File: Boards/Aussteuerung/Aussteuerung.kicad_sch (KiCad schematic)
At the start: 17 parts, among them J1 6V3_Heater, J2 Signal_R, J3 Signal_R, J4 250VDC, K1 FINDER-34.51, U1 EM84

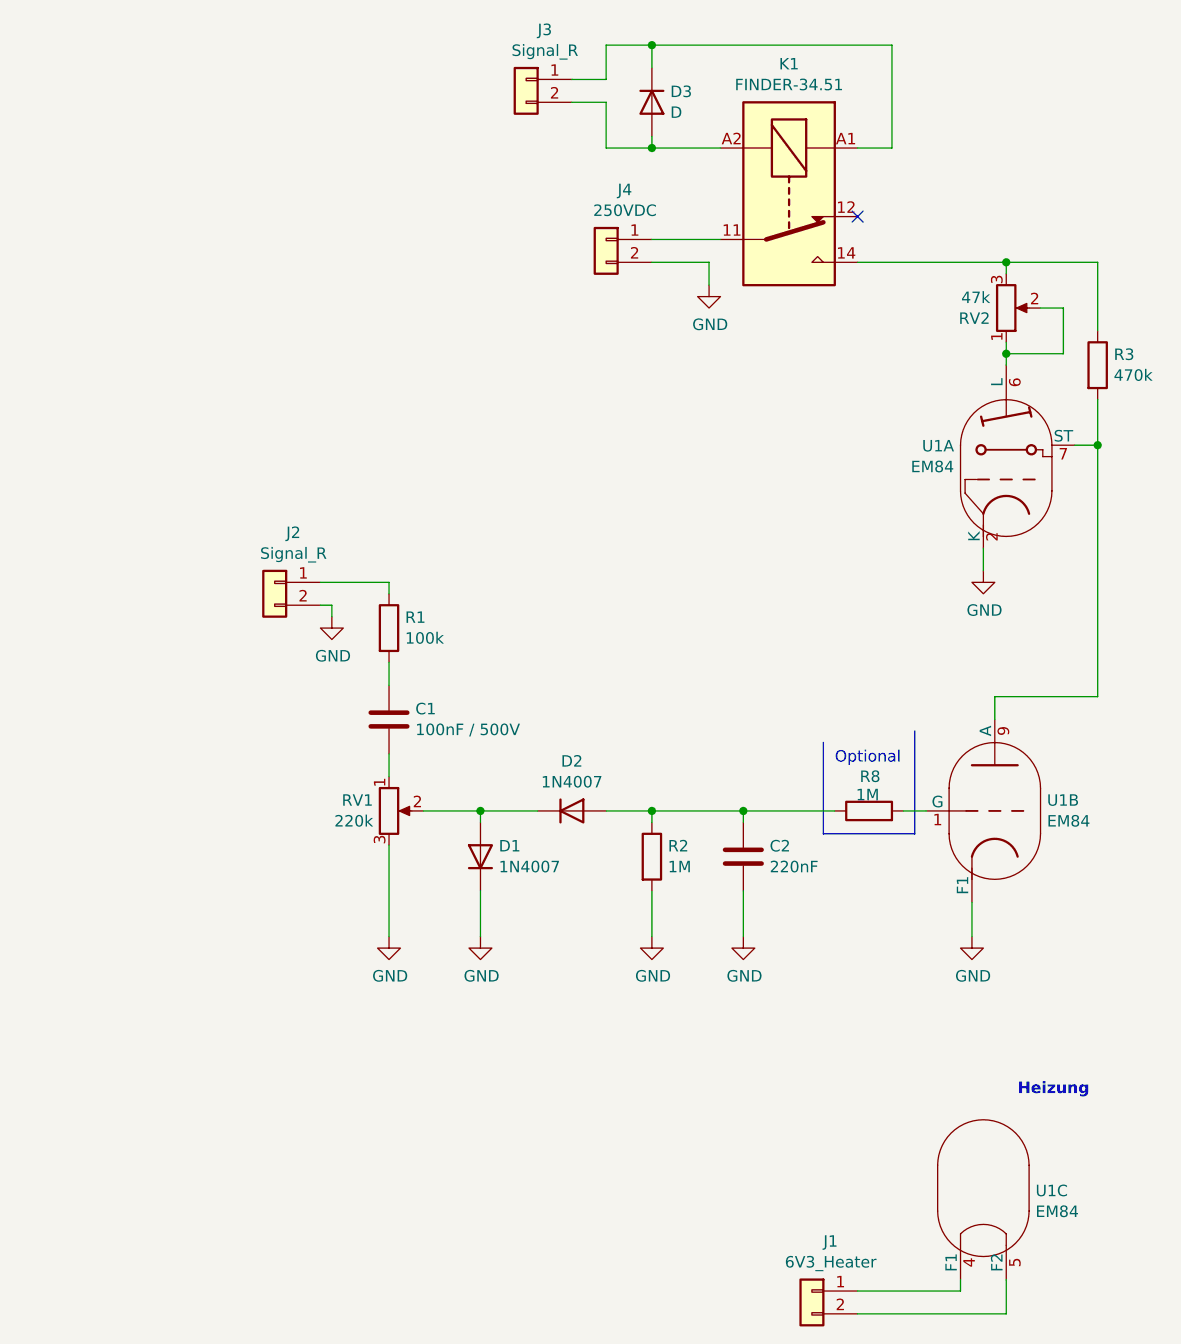
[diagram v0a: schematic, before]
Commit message: Leiterplatten erstellt
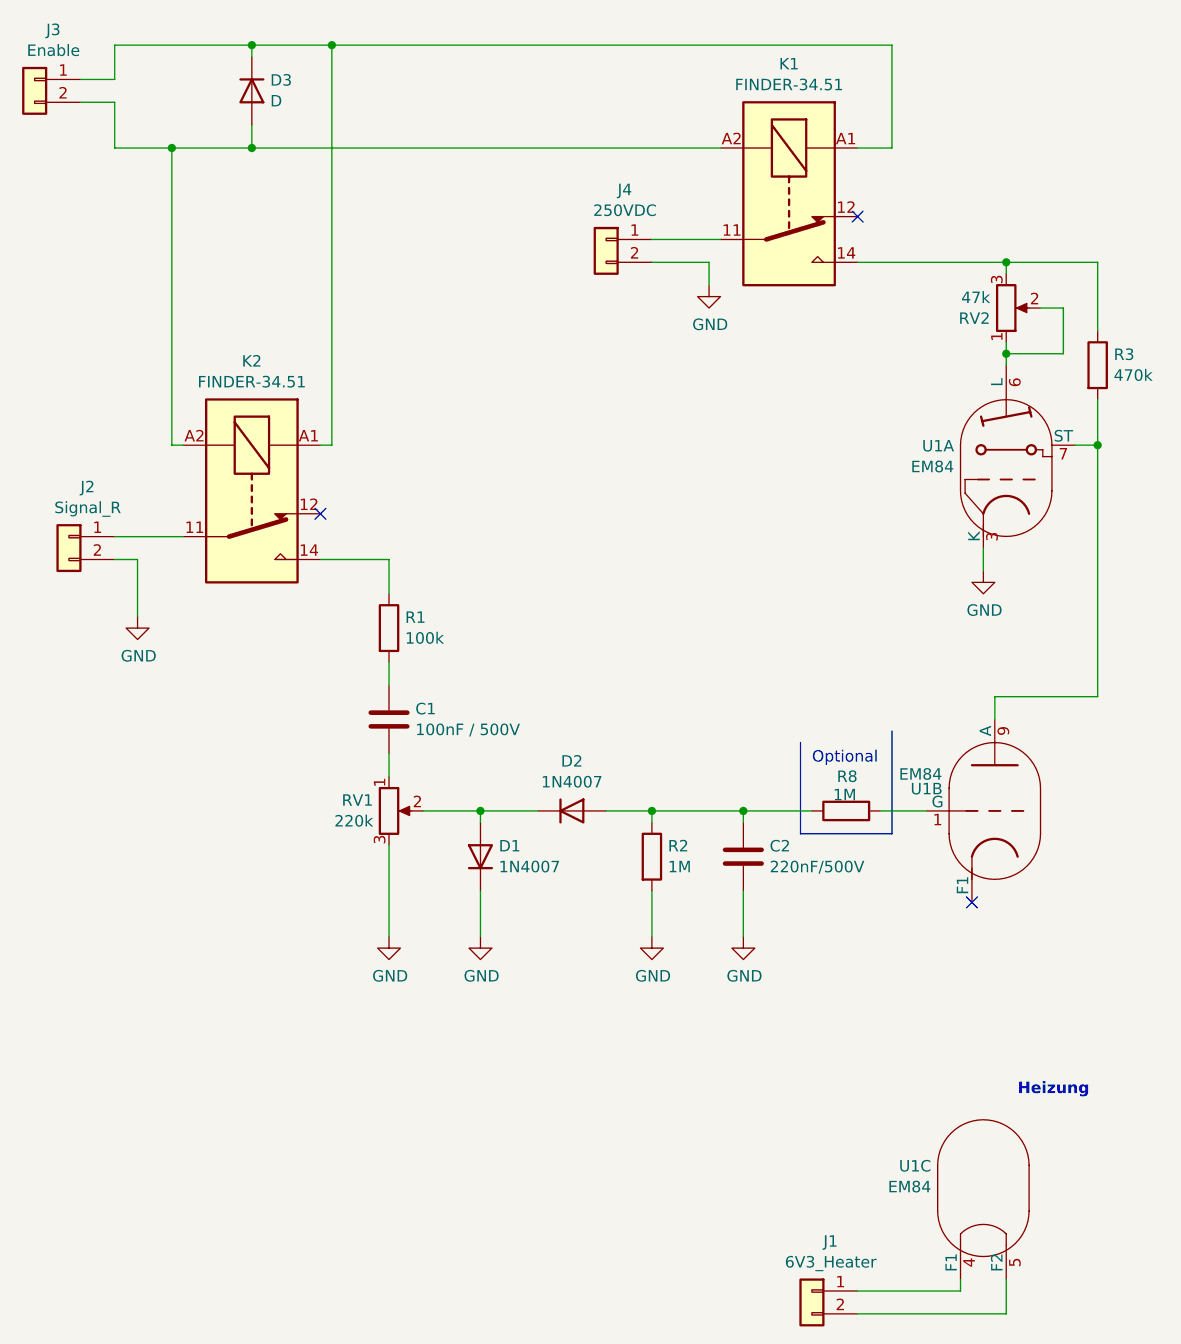
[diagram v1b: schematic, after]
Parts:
- added K2: FINDER-34.51, Relay_THT:Relay_SPDT_Finder_34.51_Vertical, symbol Relay:FINDER-34.51
- C1: footprint Capacitor_THT:C_Disc_D5.0mm_W2.5mm_P5.00mm -> Capacitor_THT:C_Rect_L26.5mm_W7.0mm_P22.50mm_MKS4
- C2: value 220nF -> 220nF/500V; footprint Capacitor_THT:C_Disc_D5.0mm_W2.5mm_P5.00mm -> Capacitor_THT:C_Rect_L26.5mm_W8.5mm_P22.50mm_MKS4
- J3: value Signal_R -> Enable
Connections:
- net GND: now also U1.3 (K); no longer U1.2 (K), U1.~ (F1)
- net at J2.1 (Pin_1): now also K2.11; no longer R1.1
- net at D3.1 (K), J3.1 (Pin_1), K1.A1: now also K2.A1
- net at D3.2 (A), J3.2 (Pin_2), K1.A2: now also K2.A2
- new net: K2.14, R1.1
- no-connect marks 1 -> 3
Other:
- moved on the sheet: D3, J2, J3, R8
